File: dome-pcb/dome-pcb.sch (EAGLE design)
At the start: 16 parts, among them K1 CQ1-12V, K5 CQ1-12V, Q1 500mA/300V, Q2 500mA/300V, U1 ESP8266_ESP-01

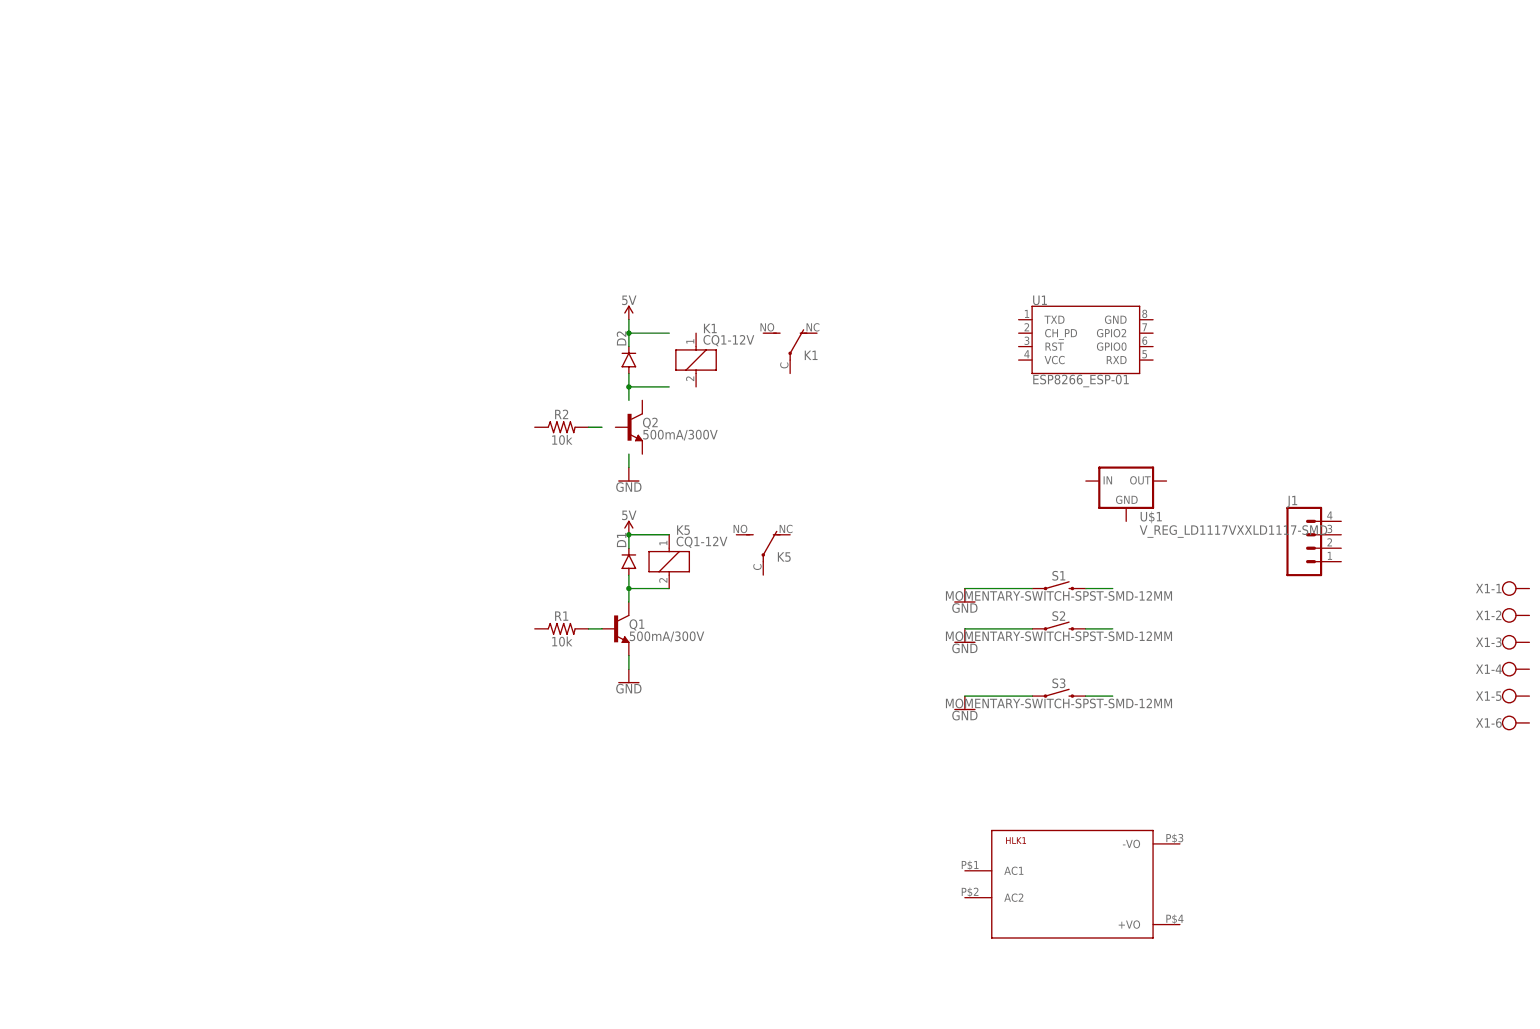
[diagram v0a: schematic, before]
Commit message: PCB Schematics and board
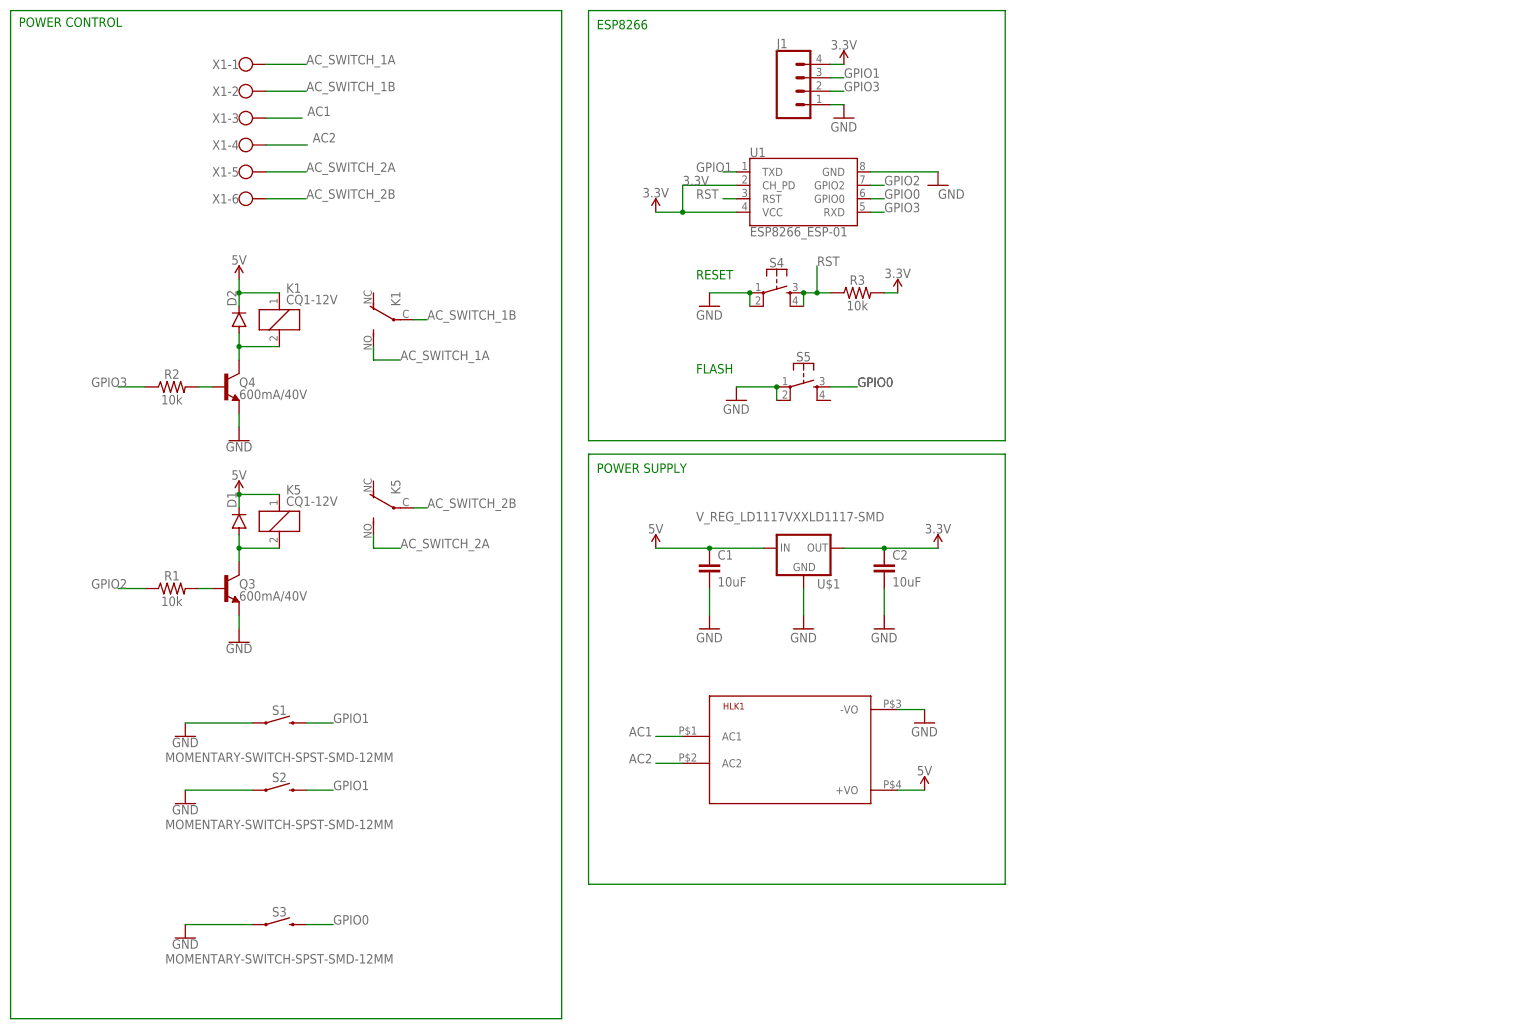
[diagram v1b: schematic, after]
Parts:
- removed Q1, Q2: 500mA/300V, DiscreteSemi:TRANS_NPN-MMBTA42
- added C1, C2: 10uF, Capacitors:10UF-0603-6.3V-20%
- added Q3, Q4: 600mA/40V, DiscreteSemi:TRANS_NPN-MMBT2222AL
- added R3: 10k, Resistors:10KOHM-0603-1/10W-1%
- added S4, S5: (no value), Switches:MOMENTARY-SWITCH-SPST-2-SMD-5.2MM
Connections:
- removed net N$1: S1.2
- removed net N$2: S2.2
- removed net N$3: S3.2
- new net 3.3V: C2.1, J1.4, R3.2, U$1.OUT, U1.CH_PD, U1.VCC
- new net AC1: HLK1.AC1, X1-3.KL
- new net AC2: HLK1.AC2, X1-4.KL
- new net AC_SWITCH_1A: K12.S, X1-1.KL
- new net AC_SWITCH_1B: K12.P, X1-2.KL
- new net AC_SWITCH_2A: K52.S, X1-5.KL
- new net AC_SWITCH_2B: K52.P, X1-6.KL
- new net GPIO0: S3.2, S5.3, U1.GPIO0
- new net GPIO1: J1.3, S1.2, S2.2, U1.TXD
- new net GPIO2: R1.1, U1.GPIO2
- new net GPIO3: J1.2, R2.1, U1.RXD
- new net RST: R3.1, S4.3, S4.4, U1.RST
- net 5V: now also C1.1, HLK1.+VO, K11.1, U$1.IN
- net GND: now also C1.2, C2.2, HLK1.-VO, J1.1, Q3.E, Q4.E, S4.1, S4.2, S5.1, S5.2, U$1.GND, U1.GND; no longer Q1.E
- net N$10: now also Q4.B
- net N$11: now also Q3.C; no longer Q1.C
- net N$12: now also Q3.B; no longer Q1.B
- net N$9: now also K11.2, Q4.C
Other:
- note added: "ESP8266"
- note added: "FLASH"
- note added: "POWER CONTROL"
- note added: "POWER SUPPLY"
- note added: "RESET"
- moved on the sheet: D1, D2, HLK1, J1, K1, K5, R1, R2, S1, S2, S3, U$1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
